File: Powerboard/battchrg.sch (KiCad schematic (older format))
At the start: 56 parts, among them J1 Thermistor Connection, Q1(ACFET) SI7617DN-T1-GE3, Q2 SI7617DN-T1-GE3, Q3 SI7617DN-T1-GE3, Q4 SIS412DN-T1-GE3, Q5 SIS412DN-T1-GE3

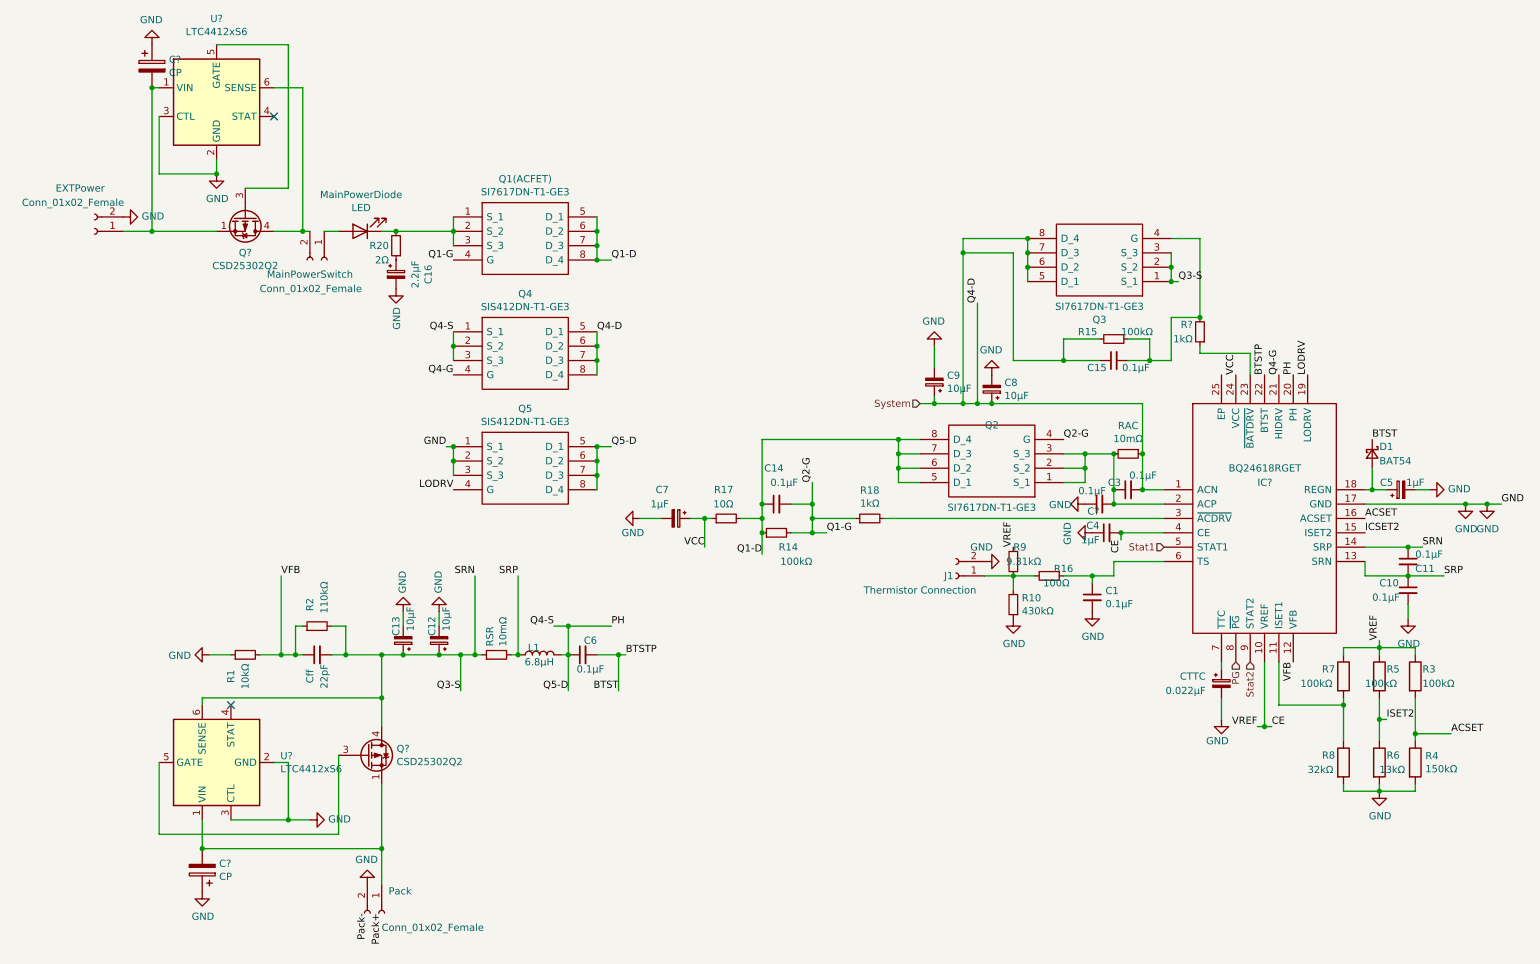
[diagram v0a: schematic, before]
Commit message: 13/02/2022
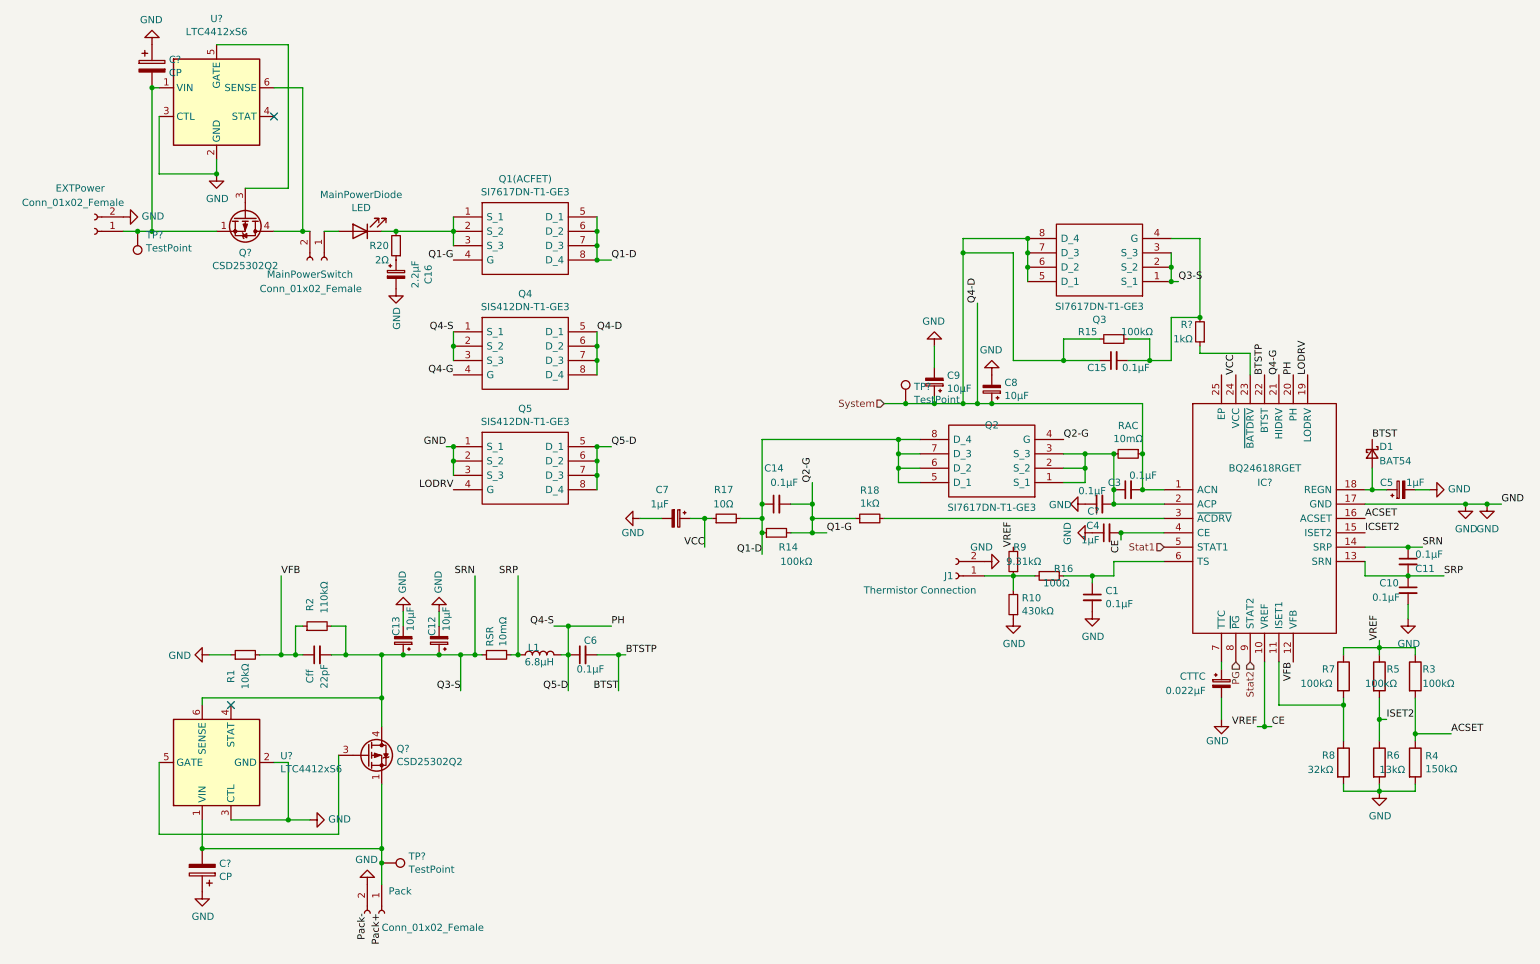
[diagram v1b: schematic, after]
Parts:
- added TP? (x3): TestPoint, symbol Connector:TestPoint
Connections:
- net System: now also TP?.1
- net at C?.2, EXTPower.1 (Pin_1), Q?.1 (S)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: now also TP?.1
- net at C?.2, Pack.1 (Pin_1), Q?.1 (S)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: now also TP?.1
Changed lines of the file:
@@
 	6650 3050 6650 3200
-Wire Wire Line
-	6550 3450 6650 3450
 Wire Wire Line
 	6650 3400 6650 3450
@@
 Text Label 4450 5450 2    50   ~ 0
 BTST
-Text HLabel 6550 3450 0    50   Input ~ 0
+Text HLabel 6300 3450 0    50   Input ~ 0
 System
 Text HLabel 8850 5250 3    50   Input ~ 0
@@
 Connection ~ 1200 2250
 Wire Wire Line
-	1200 2250 1000 2250
+	1200 2250 1100 2250
 Wire Wire Line
 	1200 2250 1650 2250
@@
 	1750 6350 2150 6350
 Wire Wire Line
-	2800 6550 2800 6800
+	2800 6550 2800 6650
 Connection ~ 2800 6550
 Wire Wire Line
@@
 	0    1    1    0
 $EndComp
+$Comp
+L Connector:TestPoint TP?
+U 1 1 620C3115
+P 1100 2250
+F 0 "TP?" H 1042 2276 50  0000 R CNN
+F 1 "TestPoint" H 1042 2367 50  0000 R CNN
+F 2 "" H 1300 2250 50  0001 C CNN
+F 3 "~" H 1300 2250 50  0001 C CNN
+	1    1100 2250
+	-1   0    0    1
+$EndComp
+Connection ~ 1100 2250
+Wire Wire Line
+	1100 2250 1000 2250
+$Comp
+L Connector:TestPoint TP?
+U 1 1 620C3E08
+P 2800 6650
+F 0 "TP?" V 2754 6838 50  0000 L CNN
+F 1 "TestPoint" V 2845 6838 50  0000 L CNN
+F 2 "" H 3000 6650 50  0001 C CNN
+F 3 "~" H 3000 6650 50  0001 C CNN
+	1    2800 6650
+	0    1    1    0
+$EndComp
+Connection ~ 2800 6650
+Wire Wire Line
+	2800 6650 2800 6800
+Wire Wire Line
+	6300 3450 6450 3450
+$Comp
+L Connector:TestPoint TP?
+U 1 1 620D1148
+P 6450 3450
+F 0 "TP?" H 6508 3568 50  0000 L CNN
+F 1 "TestPoint" H 6508 3477 50  0000 L CNN
+F 2 "" H 6650 3450 50  0001 C CNN
+F 3 "~" H 6650 3450 50  0001 C CNN
+	1    6450 3450
+	1    0    0    -1
+$EndComp
+Connection ~ 6450 3450
+Wire Wire Line
+	6450 3450 6650 3450
 $EndSCHEMATC
